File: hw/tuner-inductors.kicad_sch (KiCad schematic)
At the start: 19 parts, among them K1701 G2RL-2, K1702 G2RL-2, K1703 G2RL-2, K1704 G2RL-2, K1705 G2RL-2, K1706 G2RL-2, K1707 G2RL-2, U1701 TPIC6C595PWR

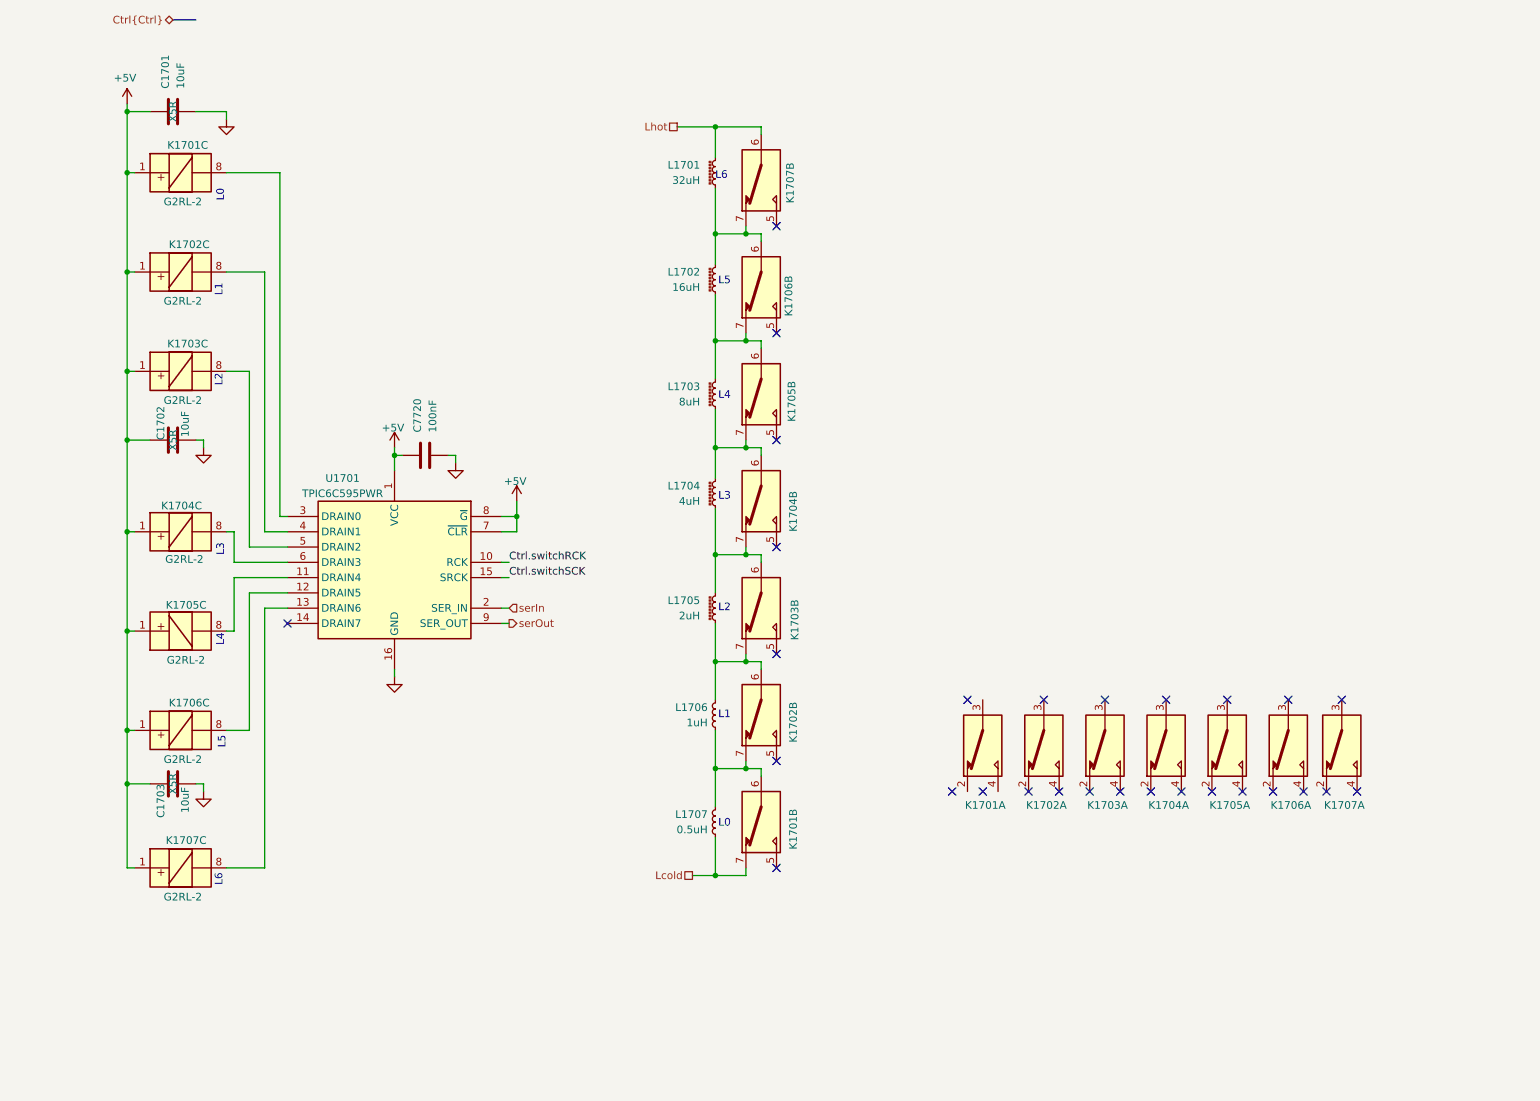
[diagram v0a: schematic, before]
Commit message: I think I have finished the relay conversion and 5V SPI I/O expander crap
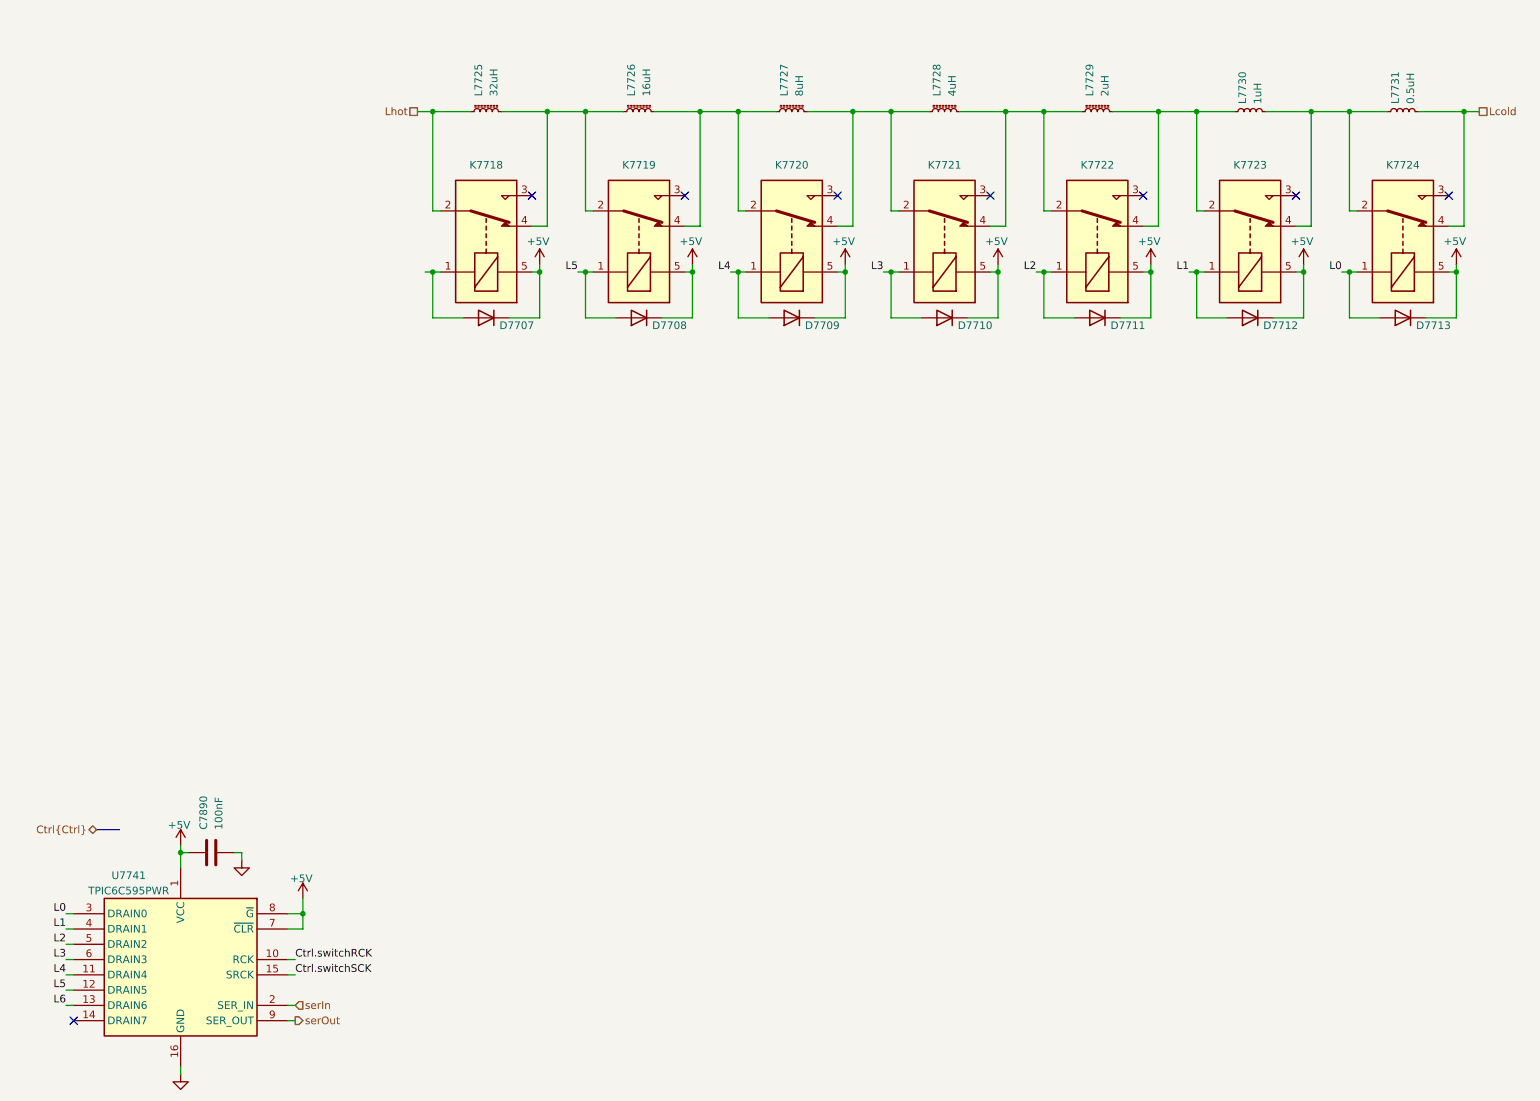
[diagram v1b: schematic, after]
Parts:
- removed C1701, C1702, C1703: 10uF, Capacitor_SMD:C_0805_2012Metric, symbol Device:C
- removed K1701, K1702, K1703, K1704, K1705, K1706, K1707: G2RL-2, Library:Relay_DPDT_Omron_G2RL-2, symbol Library:G2RL-2-functional
- removed L1706: 1uH, Library:Coilcraft-uni10, symbol Device:L_Small
- added D7707, D7708, D7709, D7710, D7711, D7712, D7713: 1N4148W, Diode_SMD:D_SOD-123, symbol Diode:1N4148W
- added K7718, K7719, K7720, K7721, K7722, K7723, K7724: G5Q-14-05, Relay_THT:Relay_SPDT_Omron-G5Q-1, symbol Relay:G5Q-1
- added L7730: 1uH, Library:Coilcraft-uni10, symbol Device:L_Small
- renumbered C7720 to C7890, L1701 to L7725, L1702 to L7726, L1703 to L7727, L1704 to L7728, L1705 to L7729, L1707 to L7731, U1701 to U7741
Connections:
- net +5V: now also D7707.1 (K), D7708.1 (K), D7709.1 (K), D7710.1 (K), D7711.1 (K), D7712.1 (K), D7713.1 (K), K7718.5, K7719.5, K7720.5, K7721.5, K7722.5, K7723.5, K7724.5
- net Lcold: now also K7724.4
- net Lhot: now also K7718.2
- net L4: now reaches U7741.11 (DRAIN4)
- net L4: now also D7709.2 (A), K7720.1
- net at L7725.2, L7726.1: now also K7718.4, K7719.2
- net at L7726.2, L7727.1: now also K7719.4, K7720.2
- net at L7728.2, L7729.1: now also K7721.4, K7722.2
- net at L7729.2: now also K7722.4, K7723.2, L7730.1
- net L6: now reaches U7741.13 (DRAIN6)
- net at L7731.1: now also K7723.4, K7724.2, L7730.2
- net at L7727.2, L7728.1: now also K7720.4, K7721.2
- net L5: now reaches U7741.12 (DRAIN5)
- net L5: now also D7708.2 (A), K7719.1
- net L0: now reaches U7741.3 (DRAIN0)
- net L0: now also D7713.2 (A), K7724.1
- net L1: now reaches U7741.4 (DRAIN1)
- net L1: now also D7712.2 (A), K7723.1
- net L2: now reaches U7741.5 (DRAIN2)
- net L2: now also D7711.2 (A), K7722.1
- net L3: now reaches U7741.6 (DRAIN3)
- net L3: now also D7710.2 (A), K7721.1
- new net: D7707.2 (A), K7718.1
- no-connect marks 29 -> 8
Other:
- note removed: "L0"
- note removed: "L1"
- note removed: "L2"
- note removed: "L3"
- note removed: "L4"
- note removed: "L5"
- note removed: "L6"
- moved on the sheet: C7890, L7725, L7726, L7727, L7728, L7729, L7731, U7741
